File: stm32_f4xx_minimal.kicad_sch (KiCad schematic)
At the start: 45 parts, among them Q1 AO3401A, SW1 SW_SPDT, U1 MP2359DJ, U2 STM32F405RGT6, U3 W25N01GVZEIG_TR, Y1 16MHz

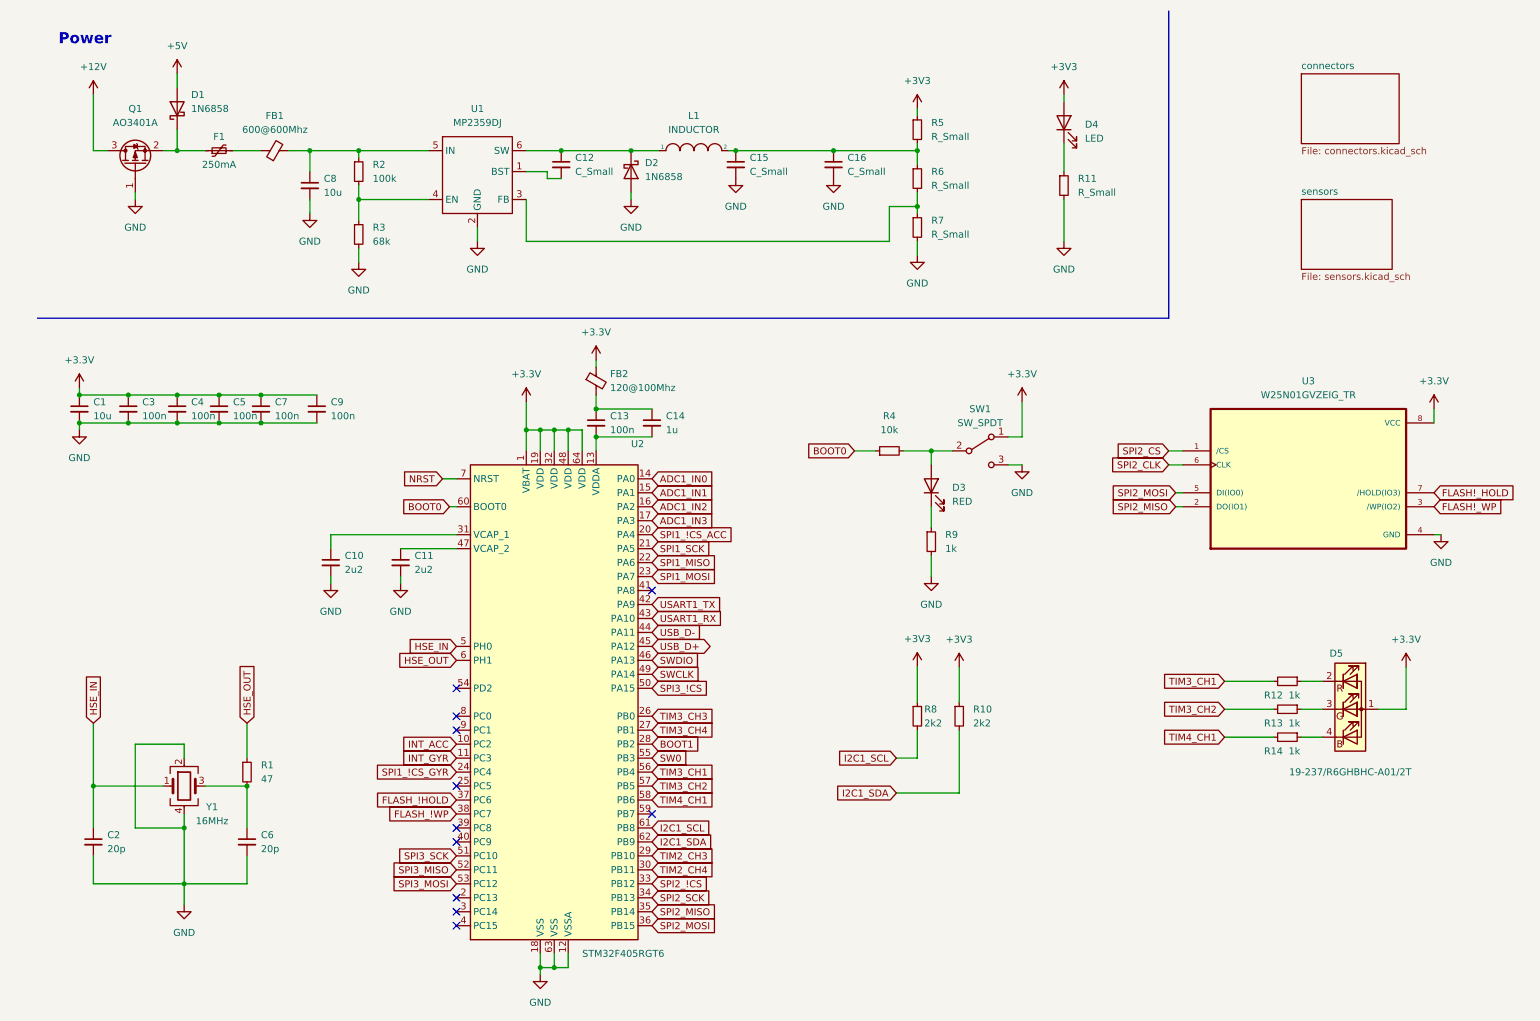
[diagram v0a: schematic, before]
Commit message: updated schematic
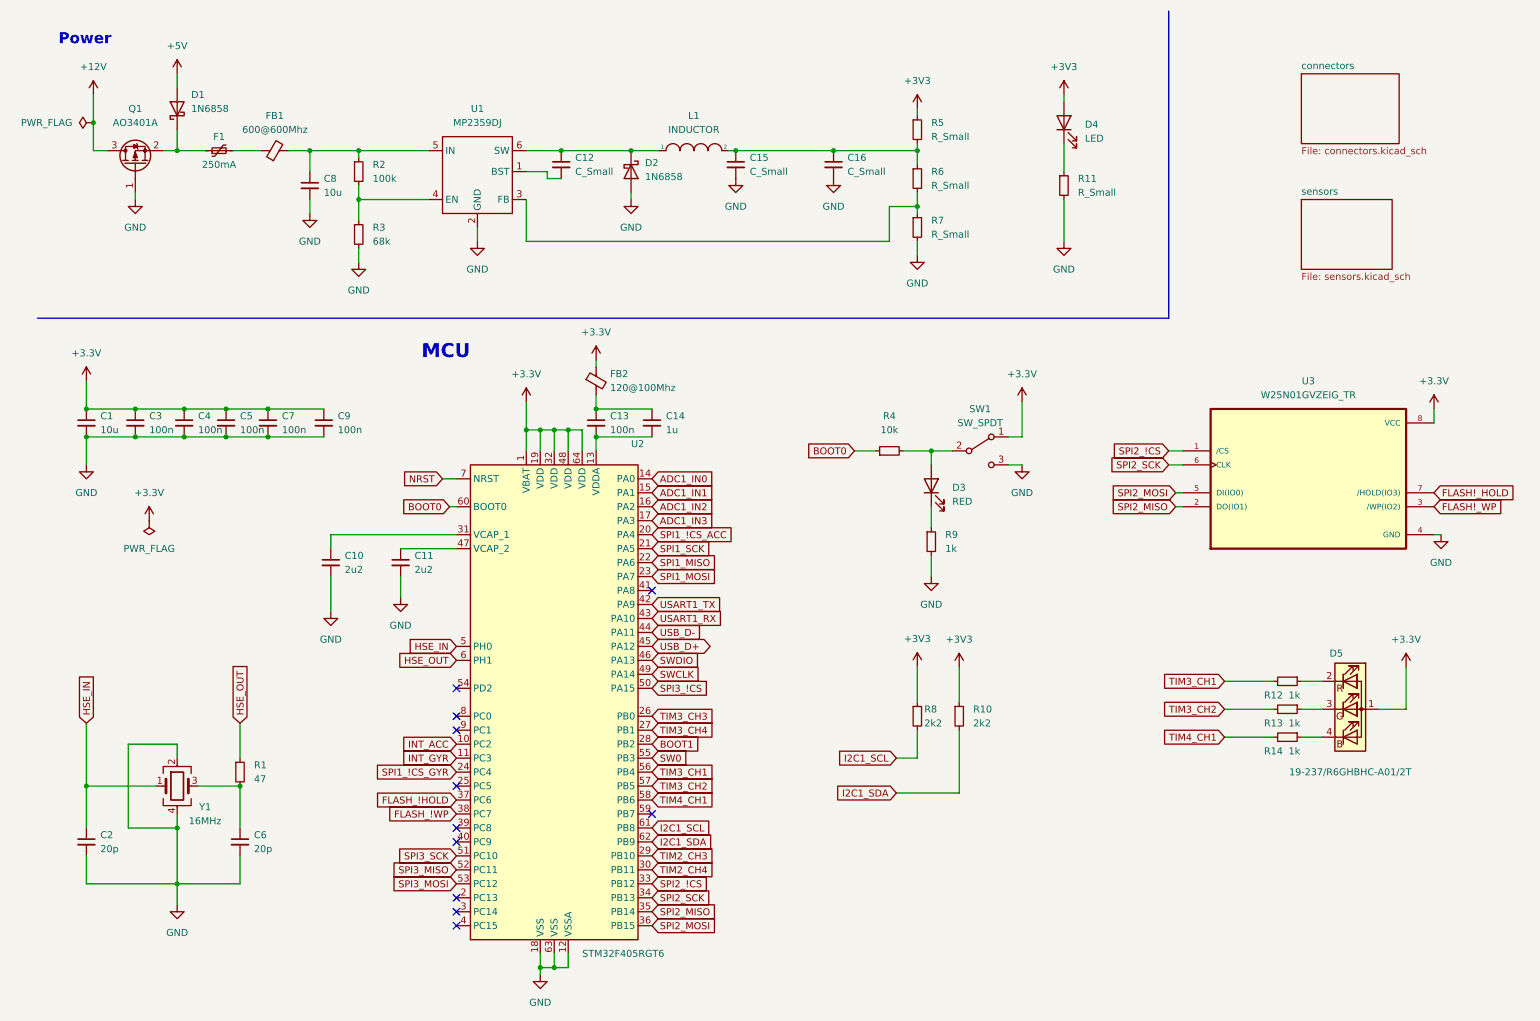
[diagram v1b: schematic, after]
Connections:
- net SPI2_CLK is gone; now on net SPI2_SCK: U3.6 (CLK)
- net SPI2_CS is gone; now on net SPI2_!CS: U3.1 (/CS)
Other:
- note added: "MCU"
- moved on the sheet: C1, C2, C3, C4, C5, C6, C7, C9, R1, Y1
